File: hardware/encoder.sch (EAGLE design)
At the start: 13 parts

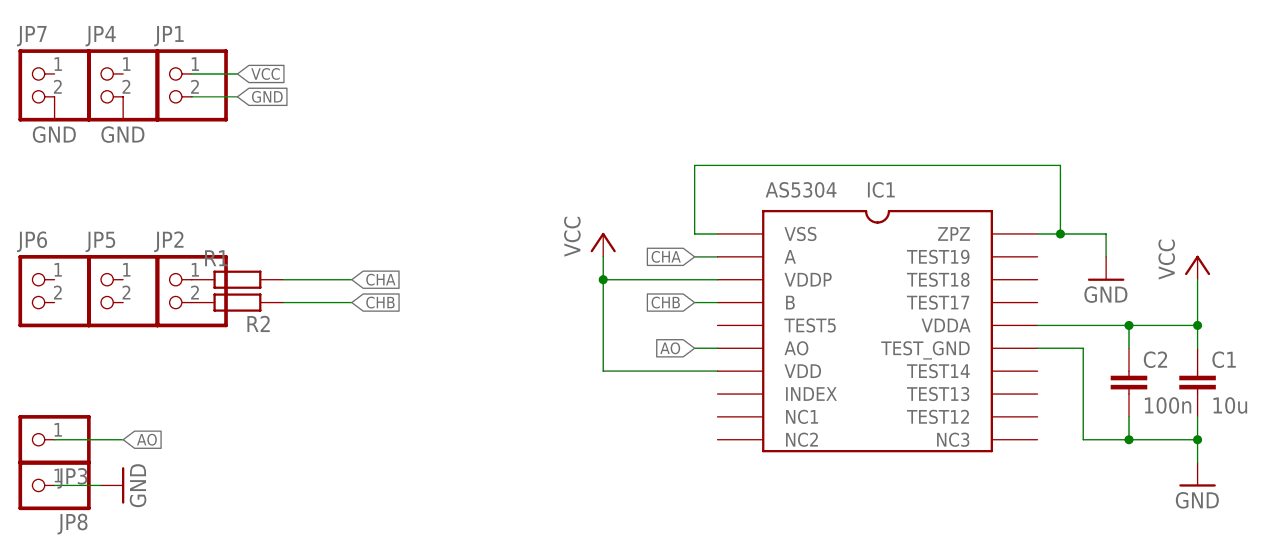
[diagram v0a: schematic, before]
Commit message: new driver
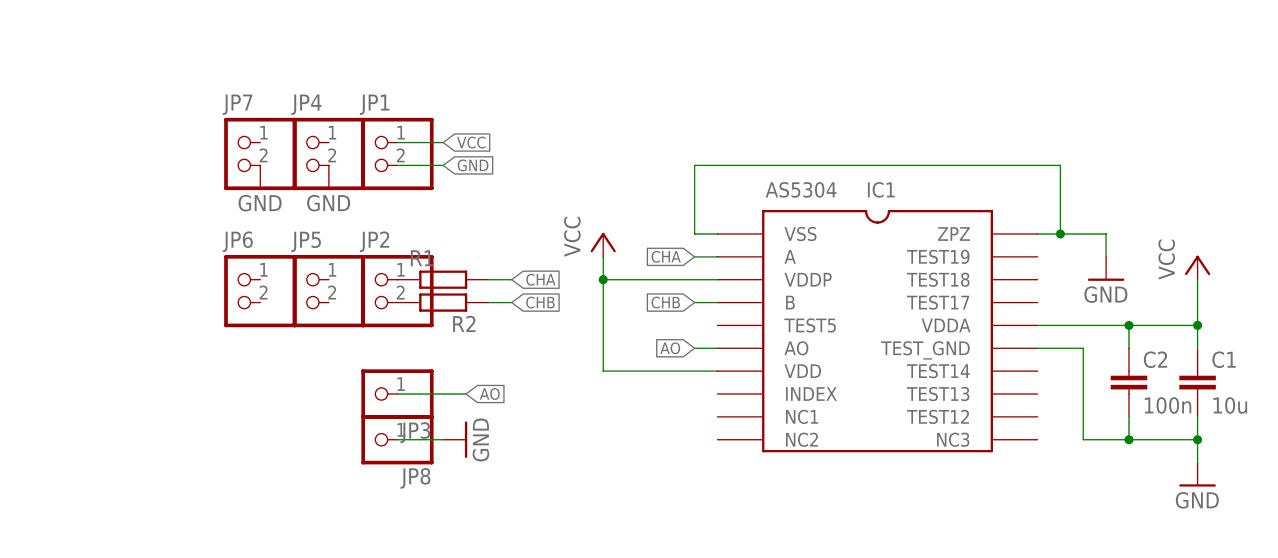
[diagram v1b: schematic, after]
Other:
- moved on the sheet: JP1, JP2, JP3, JP4, JP5, JP6, JP7, JP8, R1, R2
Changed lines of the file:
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@@
 <attribute name="VALUE" x="29.464" y="-9.779" size="1.778" layer="96"/>
 </instance>
-<instance part="JP1" gate="G$1" x="-76.2" y="26.67"/>
-<instance part="JP2" gate="G$1" x="-76.2" y="3.81"/>
-<instance part="R1" gate="G$1" x="-71.12" y="5.08"/>
-<instance part="R2" gate="G$1" x="-71.12" y="2.54" rot="R180"/>
-<instance part="JP3" gate="G$1" x="-93.98" y="-12.7" rot="R180"/>
-<instance part="JP4" gate="G$1" x="-83.82" y="26.67"/>
-<instance part="JP5" gate="G$1" x="-83.82" y="3.81"/>
-<instance part="JP8" gate="G$1" x="-93.98" y="-17.78" rot="R180"/>
-<instance part="GND3" gate="1" x="-83.82" y="-17.78" rot="R90"/>
-<instance part="GND4" gate="1" x="-83.82" y="22.86"/>
-<instance part="JP6" gate="G$1" x="-91.44" y="3.81"/>
-<instance part="JP7" gate="G$1" x="-91.44" y="26.67"/>
-<instance part="GND5" gate="1" x="-91.44" y="22.86"/>
+<instance part="JP1" gate="G$1" x="-53.34" y="19.05"/>
+<instance part="JP2" gate="G$1" x="-53.34" y="3.81"/>
+<instance part="R1" gate="G$1" x="-48.26" y="5.08"/>
+<instance part="R2" gate="G$1" x="-48.26" y="2.54" rot="R180"/>
+<instance part="JP3" gate="G$1" x="-55.88" y="-7.62" rot="R180"/>
+<instance part="JP4" gate="G$1" x="-60.96" y="19.05"/>
+<instance part="JP5" gate="G$1" x="-60.96" y="3.81"/>
+<instance part="JP8" gate="G$1" x="-55.88" y="-12.7" rot="R180"/>
+<instance part="GND3" gate="1" x="-45.72" y="-12.7" rot="R90"/>
+<instance part="GND4" gate="1" x="-60.96" y="15.24"/>
+<instance part="JP6" gate="G$1" x="-68.58" y="3.81"/>
+<instance part="JP7" gate="G$1" x="-68.58" y="19.05"/>
+<instance part="GND5" gate="1" x="-68.58" y="15.24"/>
 </instances>
 <busses>
@@
 </segment>
 <segment>
-<wire x1="-76.2" y1="25.4" x2="-71.12" y2="25.4" width="0.1524" layer="91"/>
-<label x="-71.12" y="25.4" size="1.27" layer="95" xref="yes"/>
+<wire x1="-53.34" y1="17.78" x2="-48.26" y2="17.78" width="0.1524" layer="91"/>
+<label x="-48.26" y="17.78" size="1.27" layer="95" xref="yes"/>
 <pinref part="JP1" gate="G$1" pin="2"/>
 </segment>
@@
 <pinref part="JP8" gate="G$1" pin="1"/>
 <pinref part="GND3" gate="1" pin="GND"/>
-<wire x1="-91.44" y1="-17.78" x2="-86.36" y2="-17.78" width="0.1524" layer="91"/>
+<wire x1="-53.34" y1="-12.7" x2="-48.26" y2="-12.7" width="0.1524" layer="91"/>
 </segment>
 <segment>
@@
 <segment>
 <pinref part="R1" gate="G$1" pin="2"/>
-<wire x1="-66.04" y1="5.08" x2="-58.42" y2="5.08" width="0.1524" layer="91"/>
-<label x="-58.42" y="5.08" size="1.27" layer="95" xref="yes"/>
+<wire x1="-43.18" y1="5.08" x2="-40.64" y2="5.08" width="0.1524" layer="91"/>
+<label x="-40.64" y="5.08" size="1.27" layer="95" xref="yes"/>
 </segment>
 </net>
@@
 <segment>
 <pinref part="R2" gate="G$1" pin="1"/>
-<label x="-58.42" y="2.54" size="1.27" layer="95" xref="yes"/>
-<wire x1="-66.04" y1="2.54" x2="-58.42" y2="2.54" width="0.1524" layer="91"/>
+<wire x1="-43.18" y1="2.54" x2="-40.64" y2="2.54" width="0.1524" layer="91"/>
+<label x="-40.64" y="2.54" size="1.27" layer="95" xref="yes"/>
 </segment>
 </net>
@@
 </segment>
 <segment>
-<wire x1="-76.2" y1="27.94" x2="-71.12" y2="27.94" width="0.1524" layer="91"/>
-<label x="-71.12" y="27.94" size="1.27" layer="95" xref="yes"/>
+<wire x1="-53.34" y1="20.32" x2="-48.26" y2="20.32" width="0.1524" layer="91"/>
+<label x="-48.26" y="20.32" size="1.27" layer="95" xref="yes"/>
 <pinref part="JP1" gate="G$1" pin="1"/>
 </segment>
@@
 <segment>
 <pinref part="JP3" gate="G$1" pin="1"/>
-<wire x1="-91.44" y1="-12.7" x2="-83.82" y2="-12.7" width="0.1524" layer="91"/>
-<label x="-83.82" y="-12.7" size="1.27" layer="95" xref="yes"/>
+<wire x1="-53.34" y1="-7.62" x2="-45.72" y2="-7.62" width="0.1524" layer="91"/>
+<label x="-45.72" y="-7.62" size="1.27" layer="95" xref="yes"/>
 </segment>
 </net>

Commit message: poprawilem enkodery
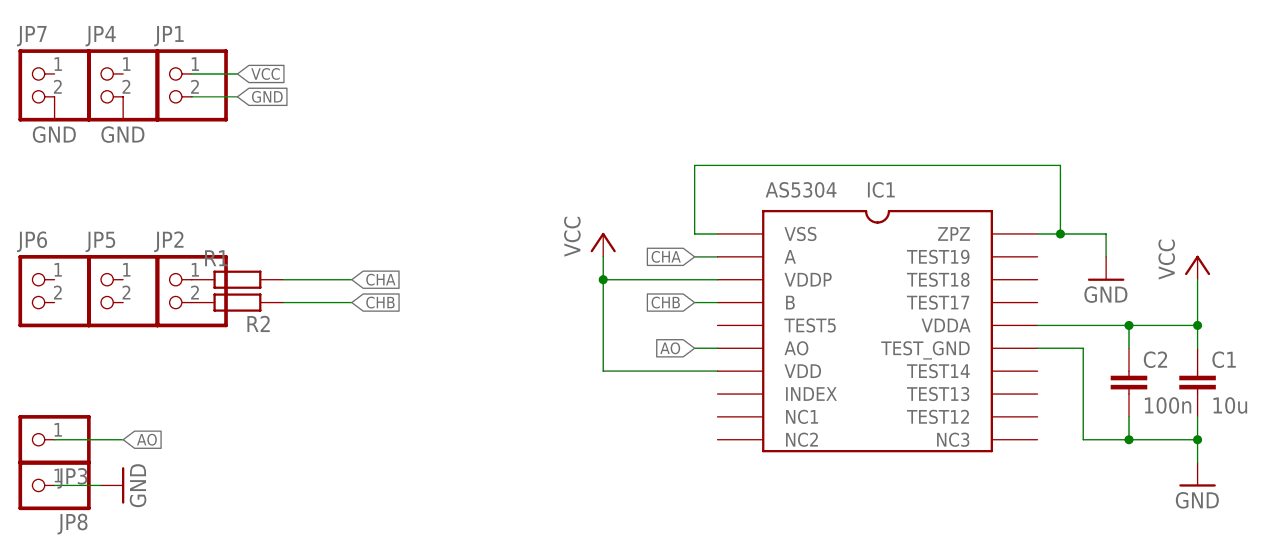
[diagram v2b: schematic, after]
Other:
- moved on the sheet: JP1, JP2, JP3, JP4, JP5, JP6, JP7, JP8, R1, R2
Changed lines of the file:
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@@
 <attribute name="VALUE" x="29.464" y="-9.779" size="1.778" layer="96"/>
 </instance>
-<instance part="JP1" gate="G$1" x="-53.34" y="19.05"/>
-<instance part="JP2" gate="G$1" x="-53.34" y="3.81"/>
-<instance part="R1" gate="G$1" x="-48.26" y="5.08"/>
-<instance part="R2" gate="G$1" x="-48.26" y="2.54" rot="R180"/>
-<instance part="JP3" gate="G$1" x="-55.88" y="-7.62" rot="R180"/>
-<instance part="JP4" gate="G$1" x="-60.96" y="19.05"/>
-<instance part="JP5" gate="G$1" x="-60.96" y="3.81"/>
-<instance part="JP8" gate="G$1" x="-55.88" y="-12.7" rot="R180"/>
-<instance part="GND3" gate="1" x="-45.72" y="-12.7" rot="R90"/>
-<instance part="GND4" gate="1" x="-60.96" y="15.24"/>
-<instance part="JP6" gate="G$1" x="-68.58" y="3.81"/>
-<instance part="JP7" gate="G$1" x="-68.58" y="19.05"/>
-<instance part="GND5" gate="1" x="-68.58" y="15.24"/>
+<instance part="JP1" gate="G$1" x="-76.2" y="26.67"/>
+<instance part="JP2" gate="G$1" x="-76.2" y="3.81"/>
+<instance part="R1" gate="G$1" x="-71.12" y="5.08"/>
+<instance part="R2" gate="G$1" x="-71.12" y="2.54" rot="R180"/>
+<instance part="JP3" gate="G$1" x="-93.98" y="-12.7" rot="R180"/>
+<instance part="JP4" gate="G$1" x="-83.82" y="26.67"/>
+<instance part="JP5" gate="G$1" x="-83.82" y="3.81"/>
+<instance part="JP8" gate="G$1" x="-93.98" y="-17.78" rot="R180"/>
+<instance part="GND3" gate="1" x="-83.82" y="-17.78" rot="R90"/>
+<instance part="GND4" gate="1" x="-83.82" y="22.86"/>
+<instance part="JP6" gate="G$1" x="-91.44" y="3.81"/>
+<instance part="JP7" gate="G$1" x="-91.44" y="26.67"/>
+<instance part="GND5" gate="1" x="-91.44" y="22.86"/>
 </instances>
 <busses>
@@
 </segment>
 <segment>
-<wire x1="-53.34" y1="17.78" x2="-48.26" y2="17.78" width="0.1524" layer="91"/>
-<label x="-48.26" y="17.78" size="1.27" layer="95" xref="yes"/>
+<wire x1="-76.2" y1="25.4" x2="-71.12" y2="25.4" width="0.1524" layer="91"/>
+<label x="-71.12" y="25.4" size="1.27" layer="95" xref="yes"/>
 <pinref part="JP1" gate="G$1" pin="2"/>
 </segment>
@@
 <pinref part="JP8" gate="G$1" pin="1"/>
 <pinref part="GND3" gate="1" pin="GND"/>
-<wire x1="-53.34" y1="-12.7" x2="-48.26" y2="-12.7" width="0.1524" layer="91"/>
+<wire x1="-91.44" y1="-17.78" x2="-86.36" y2="-17.78" width="0.1524" layer="91"/>
 </segment>
 <segment>
@@
 <segment>
 <pinref part="R1" gate="G$1" pin="2"/>
-<wire x1="-43.18" y1="5.08" x2="-40.64" y2="5.08" width="0.1524" layer="91"/>
-<label x="-40.64" y="5.08" size="1.27" layer="95" xref="yes"/>
+<wire x1="-66.04" y1="5.08" x2="-58.42" y2="5.08" width="0.1524" layer="91"/>
+<label x="-58.42" y="5.08" size="1.27" layer="95" xref="yes"/>
 </segment>
 </net>
@@
 <segment>
 <pinref part="R2" gate="G$1" pin="1"/>
-<wire x1="-43.18" y1="2.54" x2="-40.64" y2="2.54" width="0.1524" layer="91"/>
-<label x="-40.64" y="2.54" size="1.27" layer="95" xref="yes"/>
+<label x="-58.42" y="2.54" size="1.27" layer="95" xref="yes"/>
+<wire x1="-66.04" y1="2.54" x2="-58.42" y2="2.54" width="0.1524" layer="91"/>
 </segment>
 </net>
@@
 </segment>
 <segment>
-<wire x1="-53.34" y1="20.32" x2="-48.26" y2="20.32" width="0.1524" layer="91"/>
-<label x="-48.26" y="20.32" size="1.27" layer="95" xref="yes"/>
+<wire x1="-76.2" y1="27.94" x2="-71.12" y2="27.94" width="0.1524" layer="91"/>
+<label x="-71.12" y="27.94" size="1.27" layer="95" xref="yes"/>
 <pinref part="JP1" gate="G$1" pin="1"/>
 </segment>
@@
 <segment>
 <pinref part="JP3" gate="G$1" pin="1"/>
-<wire x1="-53.34" y1="-7.62" x2="-45.72" y2="-7.62" width="0.1524" layer="91"/>
-<label x="-45.72" y="-7.62" size="1.27" layer="95" xref="yes"/>
+<wire x1="-91.44" y1="-12.7" x2="-83.82" y2="-12.7" width="0.1524" layer="91"/>
+<label x="-83.82" y="-12.7" size="1.27" layer="95" xref="yes"/>
 </segment>
 </net>
